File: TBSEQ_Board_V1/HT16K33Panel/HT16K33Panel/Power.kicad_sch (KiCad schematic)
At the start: 1 part, among them J2 Conn_01x02_Socket

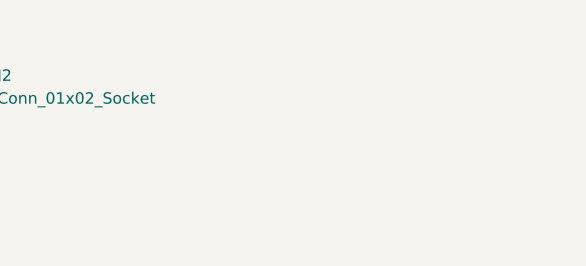
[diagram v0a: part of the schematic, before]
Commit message: HT16K33Panel DRC gaber
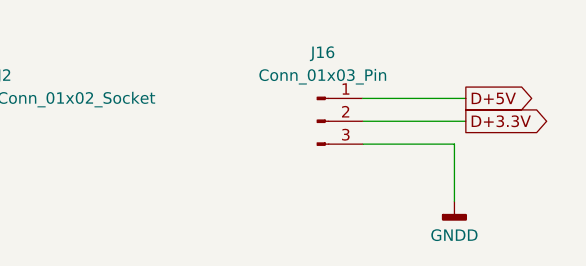
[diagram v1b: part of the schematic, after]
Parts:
- added J16: Conn_01x03_Pin, Connector_PinSocket_2.54mm:PinSocket_1x03_P2.54mm_Vertical, symbol Connector:Conn_01x03_Pin
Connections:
- net D+3.3V: now also J16.2 (Pin_2)
- net D+5V: now also J16.1 (Pin_1)
- net GNDD: now also J16.3 (Pin_3)
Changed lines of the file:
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@@
+	(wire
+		(pts
+			(xy 162.56 31.75) (xy 151.13 31.75)
+		)
+		(stroke
+			(width 0)
+			(type default)
+		)
+	)
+	(wire
+		(pts
+			(xy 161.29 36.83) (xy 151.13 36.83)
+		)
+		(stroke
+			(width 0)
+			(type default)
+		)
+	)
 	(wire
 		(pts
@@
 		(pts
 			(xy 35.56 31.75) (xy 31.75 31.75)
+		)
+		(stroke
+			(width 0)
+			(type default)
+		)
+	)
+	(wire
+		(pts
+			(xy 161.29 43.18) (xy 161.29 36.83)
+		)
+		(stroke
+			(width 0)
+			(type default)
+		)
+	)
+	(wire
+		(pts
+			(xy 162.56 34.29) (xy 151.13 34.29)
 		)
 		(stroke
@@
 		)
 	)
+	(global_label "D+3.3V"
+		(shape output)
+		(at 162.56 34.29 0)
+		(fields_autoplaced yes)
+		(effects
+			(font
+				(size 1.27 1.27)
+			)
+			(justify left)
+		)
+		(property "Intersheetrefs" "${INTERSHEET_REFS}"
+			(at 172.5 34.29 0)
+			(effects
+				(font
+					(size 1.27 1.27)
+				)
+				(justify left)
+				(hide yes)
+			)
+		)
+	)
 	(global_label "D+5V"
 		(shape output)
@@
 		(property "Intersheetrefs" "${INTERSHEET_REFS}"
 			(at 58.9257 31.75 0)
+			(effects
+				(font
+					(size 1.27 1.27)
+				)
+				(justify left)
+				(hide yes)
+			)
+		)
+	)
+	(global_label "D+5V"
+		(shape output)
+		(at 162.56 31.75 0)
+		(fields_autoplaced yes)
+		(effects
+			(font
+				(size 1.27 1.27)
+			)
+			(justify left)
+		)
+		(property "Intersheetrefs" "${INTERSHEET_REFS}"
+			(at 170.6857 31.75 0)
 			(effects
 				(font
@@
 					(unit 1)
 				)
+			)
+		)
+	)
+	(symbol
+		(lib_id "Connector:Conn_01x03_Pin")
+		(at 146.05 34.29 0)
+		(unit 1)
+		(exclude_from_sim no)
+		(in_bom yes)
+		(on_board yes)
+		(dnp no)
+		(fields_autoplaced yes)
+		(property "Reference" "J16"
+			(at 146.685 26.67 0)
+			(effects
+				(font
+					(size 1.27 1.27)
+				)
+			)
+		)
+		(property "Value" "Conn_01x03_Pin"
+			(at 146.685 29.21 0)
+			(effects
+				(font
+					(size 1.27 1.27)
+				)
+			)
+		)
+		(property "Footprint" "Connector_PinSocket_2.54mm:PinSocket_1x03_P2.54mm_Vertical"
+			(at 146.05 34.29 0)
+			(effects
+				(font
+					(size 1.27 1.27)
+				)
+				(hide yes)
+			)
+		)
+		(property "Datasheet" "~"
+			(at 146.05 34.29 0)
+			(effects
+				(font
+					(size 1.27 1.27)
+				)
+				(hide yes)
+			)
+		)
+		(property "Description" "Generic connector, single row, 01x03, script generated"
+			(at 146.05 34.29 0)
+			(effects
+				(font
+					(size 1.27 1.27)
+				)
+				(hide yes)
+			)
+		)
+		(pin "3"
+		)
+		(pin "1"
+		)
+		(pin "2"
+		)
+		(instances
+			(project "HT16K33Panel"
+				(path "/2a3172f4-85fe-4c47-84d4-31ed69e3089f/90303121-4348-4bf8-ada4-62b343a95dee"
+					(reference "J16")
+					(unit 1)
+				)
+			)
+		)
+	)
+	(symbol
+		(lib_id "power:GNDD")
+		(at 161.29 43.18 0)
+		(unit 1)
+		(exclude_from_sim no)
+		(in_bom yes)
+		(on_board yes)
+		(dnp no)
+		(property "Reference" "#PWR023"
+			(at 161.29 49.53 0)
+			(effects
+				(font
+					(size 1.27 1.27)
+				)
+				(hide yes)
+			)
+		)
+		(property "Value" "GNDD"
+			(at 161.29 46.99 0)
+			(effects
+				(font
+					(size 1.27 1.27)
+				)
+			)
+		)
+		(property "Footprint" ""
+			(at 161.29 43.18 0)
+			(effects
+				(font
+					(size 1.27 1.27)
+				)
+				(hide yes)
+			)
+		)
+		(property "Datasheet" ""
+			(at 161.29 43.18 0)
+			(effects
+				(font
+					(size 1.27 1.27)
+				)
+				(hide yes)
+			)
+		)
+		(property "Description" "Power symbol creates a global label with name \"GNDD\" , digital ground"
+			(at 161.29 43.18 0)
+			(effects
+				(font
+					(size 1.27 1.27)
+				)
+				(hide yes)
+			)
+		)
+		(pin "1"
+		)
+		(instances
+			(project "HT16K33Panel"
+				(path "/2a3172f4-85fe-4c47-84d4-31ed69e3089f/90303121-4348-4bf8-ada4-62b343a95dee"
+					(reference "#PWR023")
+					(unit 1)
+				)
